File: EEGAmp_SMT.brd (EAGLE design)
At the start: 30 x 21.6 mm, 14 parts, among them U1 TL084BCN

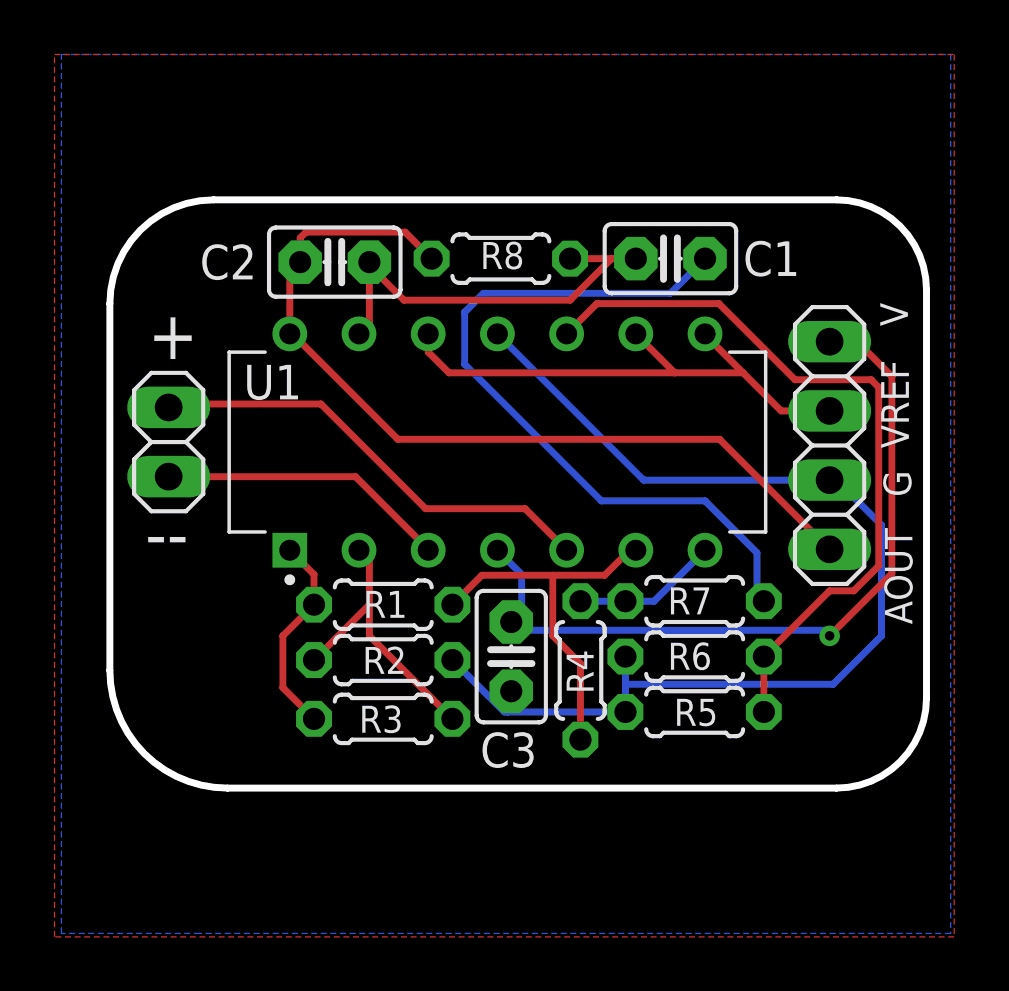
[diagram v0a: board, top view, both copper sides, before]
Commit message: smt version
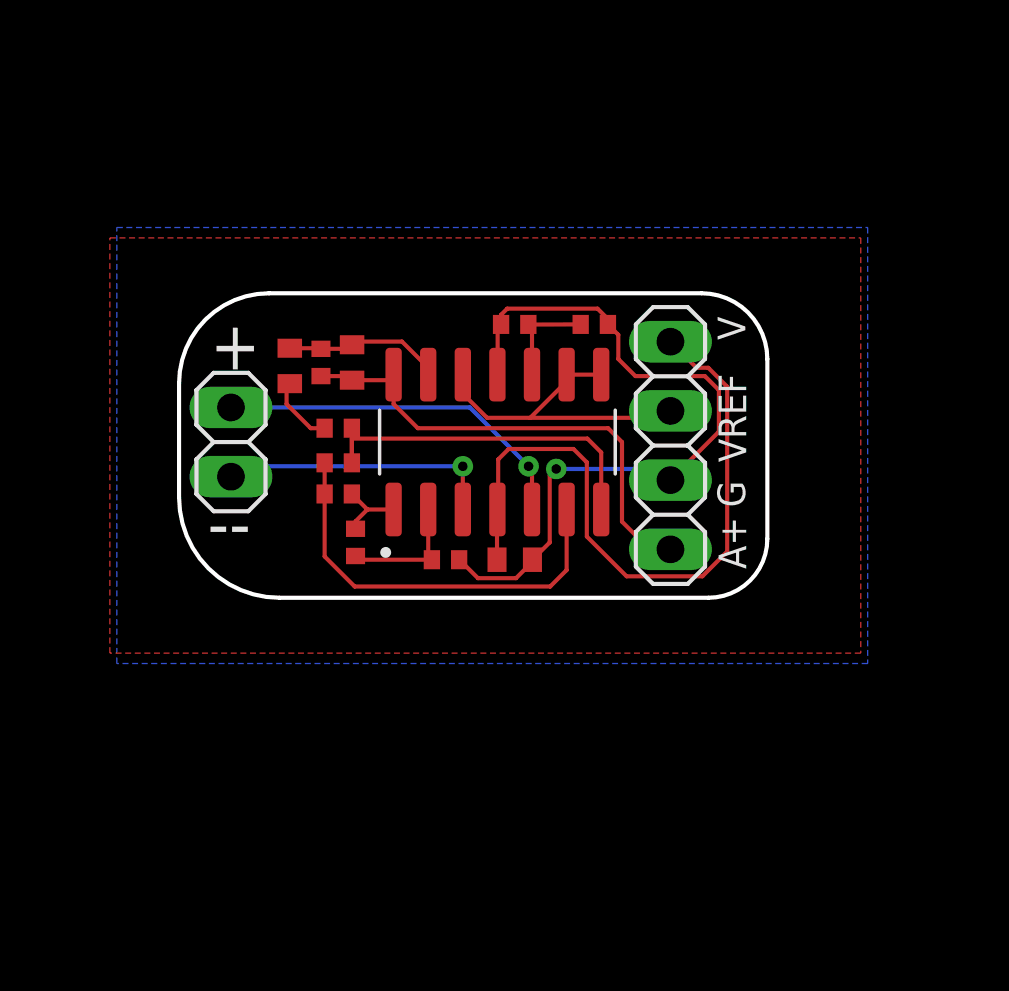
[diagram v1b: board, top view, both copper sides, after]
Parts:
- C1, C2, C3: device capacitor-wima:C2.5-2 -> rcl:C0402
- R1, R2, R3, R4, R5, R6, R7, R8: device rcl:0204/5 -> rcl:R0402
- U1: value TL084BCN -> TL084QD; device TL084BCN:DIP794W45P254L1969H508Q14 -> TL084QD:SOIC127P600X175-14N
- moved R5 14.7 mm to (30.2, 29.7), turned to 0 degrees
- moved R7 14.5 mm to (20.8, 25.9), turned to 180 degrees
- moved C1 14.5 mm to (19.1, 28.2), turned to 90 degrees
- moved R6 13.9 mm to (27.3, 29.7)
- moved R4 11.7 mm to (20.8, 24.6), turned to 0 degrees
- moved R8 7.62 mm to (20.2, 28.3), turned to 270 degrees
- moved R3 6.56 mm to (21.5, 21.7), turned to 90 degrees
- moved JP2 5.84 mm to (33.0, 25.3)
- moved R1 4.39 mm to (20.8, 23.5), turned to 180 degrees
- moved R2 4.33 mm to (24.8, 21.1)
- moved C2 3.74 mm to (21.3, 28.3), turned to 270 degrees
- moved C3 3.56 mm to (27.3, 21.1), turned to 180 degrees
- moved JP1 2.29 mm to (16.9, 25.4)
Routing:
- net N$9: track 27.0 -> 2.56 mm
- net 3IN+: track 27.4 -> 3.82 mm
- net AOUT: track 32.1 -> 18.0 mm
- net GND: track 41.6 -> 27.6 mm, vias 0 -> 1
- net 4IN-: track 16.3 -> 5.85 mm
- net VOD: track 5.35 -> 13.6 mm
- net VREF: track 20.3 -> 12.2 mm
- net 1IN-: track 10.5 -> 4.76 mm
- net 1OUT: track 7.51 -> 2.86 mm
- net VDD: track 28.5 -> 25.0 mm, vias 1 -> 0
- net AIN+: track 16.9 -> 13.5 mm, vias 0 -> 1
- net 2IN-: track 14.0 -> 15.2 mm
- net AIN-: track 10.7 -> 10.3 mm, vias 0 -> 1
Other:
- board size 30 x 21.6 mm -> 21.6 x 11.2 mm
- board text added: "A+"
- board text removed: "AOUT"
